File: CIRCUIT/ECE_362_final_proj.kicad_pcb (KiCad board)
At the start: 2 copper layers, 142.9 x 75 mm, 29 parts, among them J1 Conn_01x01_Pin, J2 Conn_01x01_Pin, J3 Conn_01x28_Socket, J4 Conn_01x28_Socket, SW2 BUTTON_MODE, SW4 BUTTON_CAPTURE, U1 TL084

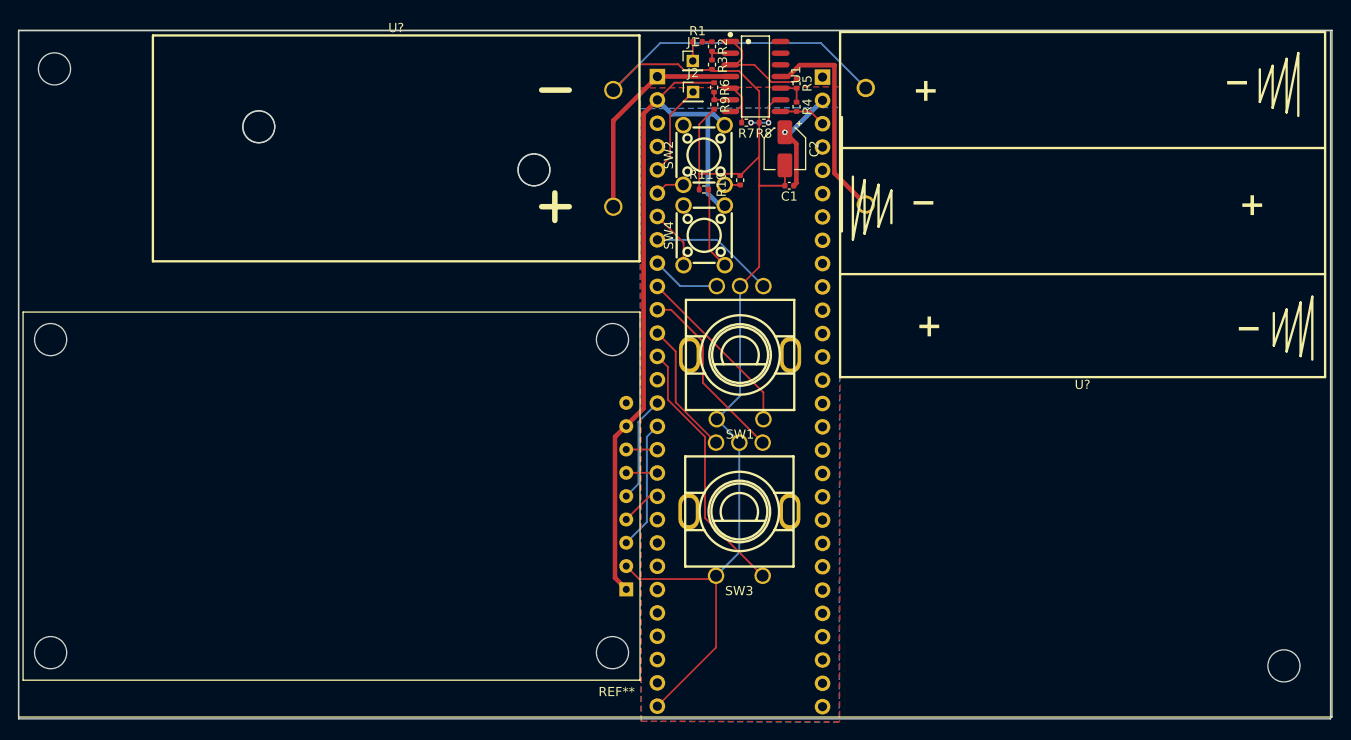
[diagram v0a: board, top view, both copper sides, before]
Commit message: rearranged board
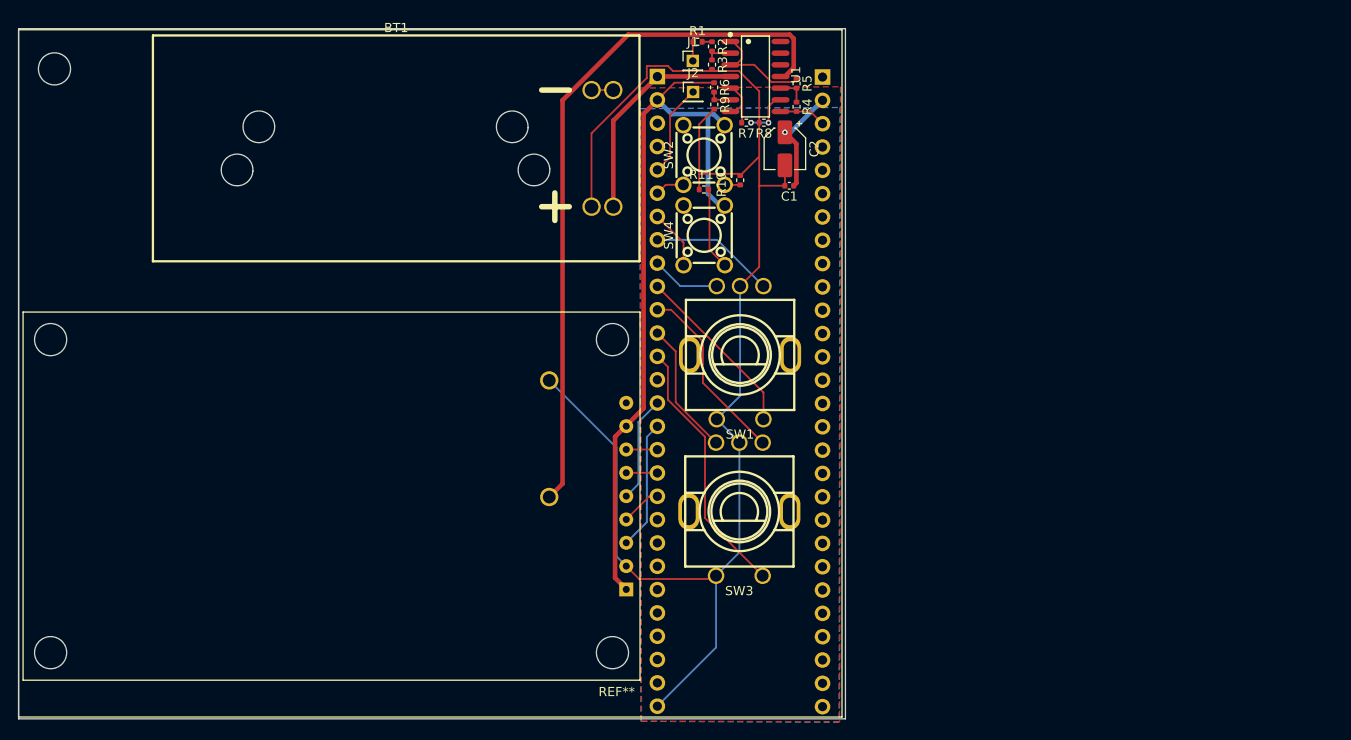
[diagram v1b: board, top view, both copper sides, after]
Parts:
- removed the ? at (-42.2, 11.9)
- removed the ? at (69.4, 70.6)
- removed the ? at (-12.3, 16.6)
- added BT2: BAT-TH_2P-L53.0-W24.6-P12.70_2468, cell_holder_3AA:BAT-TH_2P-L53.0-W24.6-P12.70_2468, B.Cu at (-6.00, 14.3)
- U?: moved to B.Cu
- moved U? 46.9 mm to (-10.6, 45.9), turned to 0 degrees
- gave numbers to parts that had none: 1
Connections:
- BT1 pad 1: GND -> BT1_GND
- REF** pad 9: x -> (no net)
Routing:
- net -BATT: track 23.0 -> 77.1 mm
- net GND: track 156.2 -> 161.8 mm
- net BT1_GND: track 0.00 -> 1.97 mm
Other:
- board size 142.9 x 75 mm -> 90.1 x 75.2 mm
